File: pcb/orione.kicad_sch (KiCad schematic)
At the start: 187 parts, among them J1 Conn_02x10_Odd_Even, J2 Conn_02x10_Odd_Even

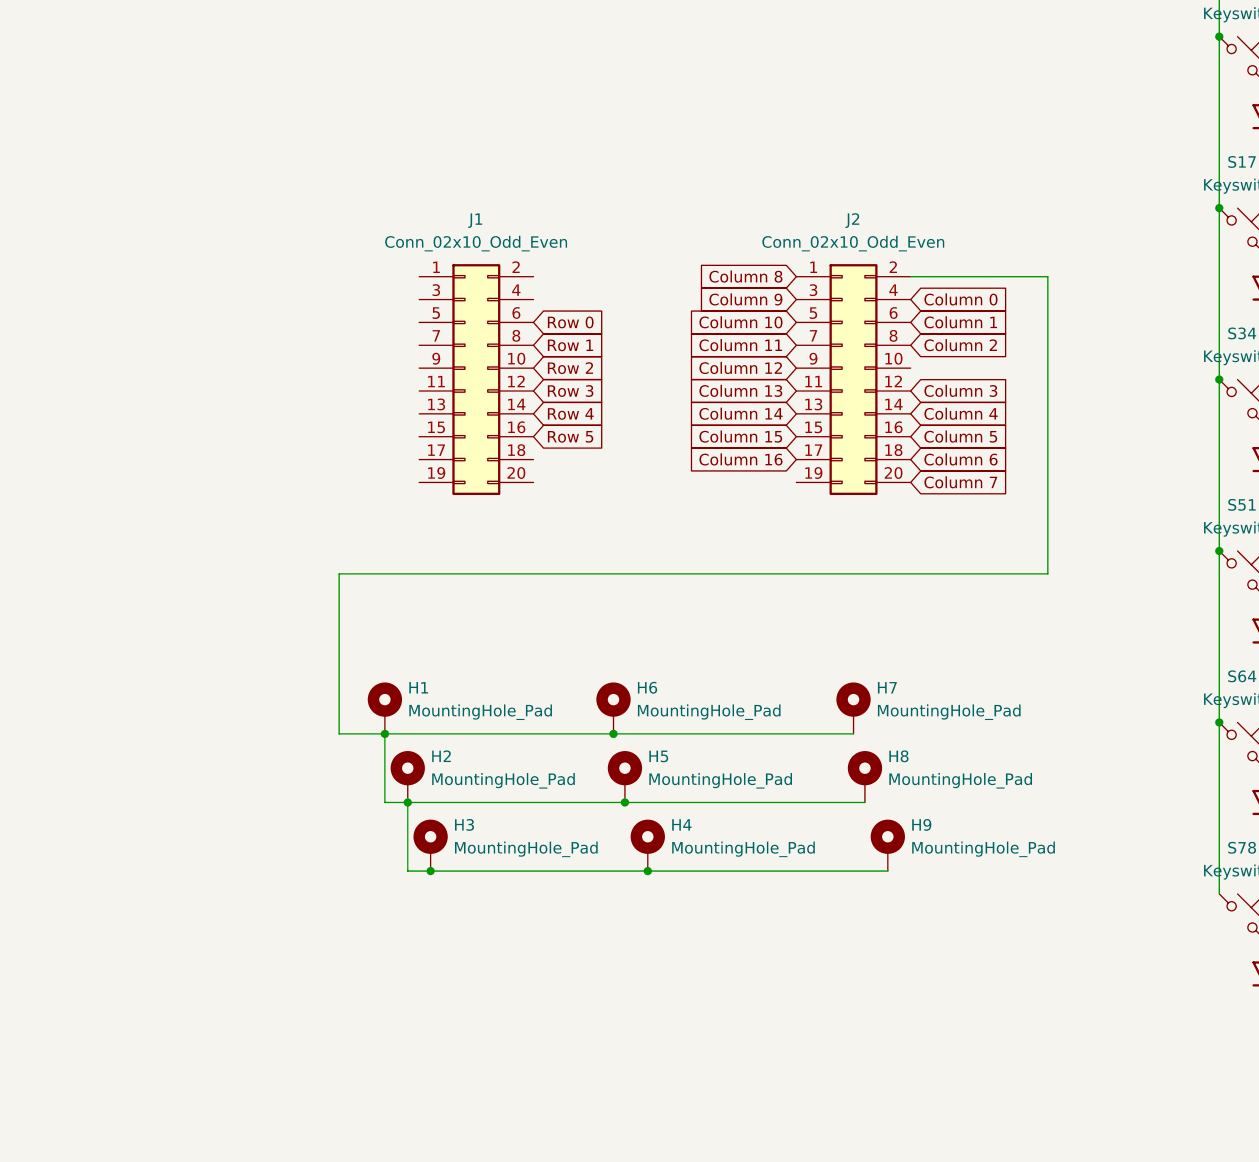
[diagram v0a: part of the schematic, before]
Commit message: minor updtaes to pcb
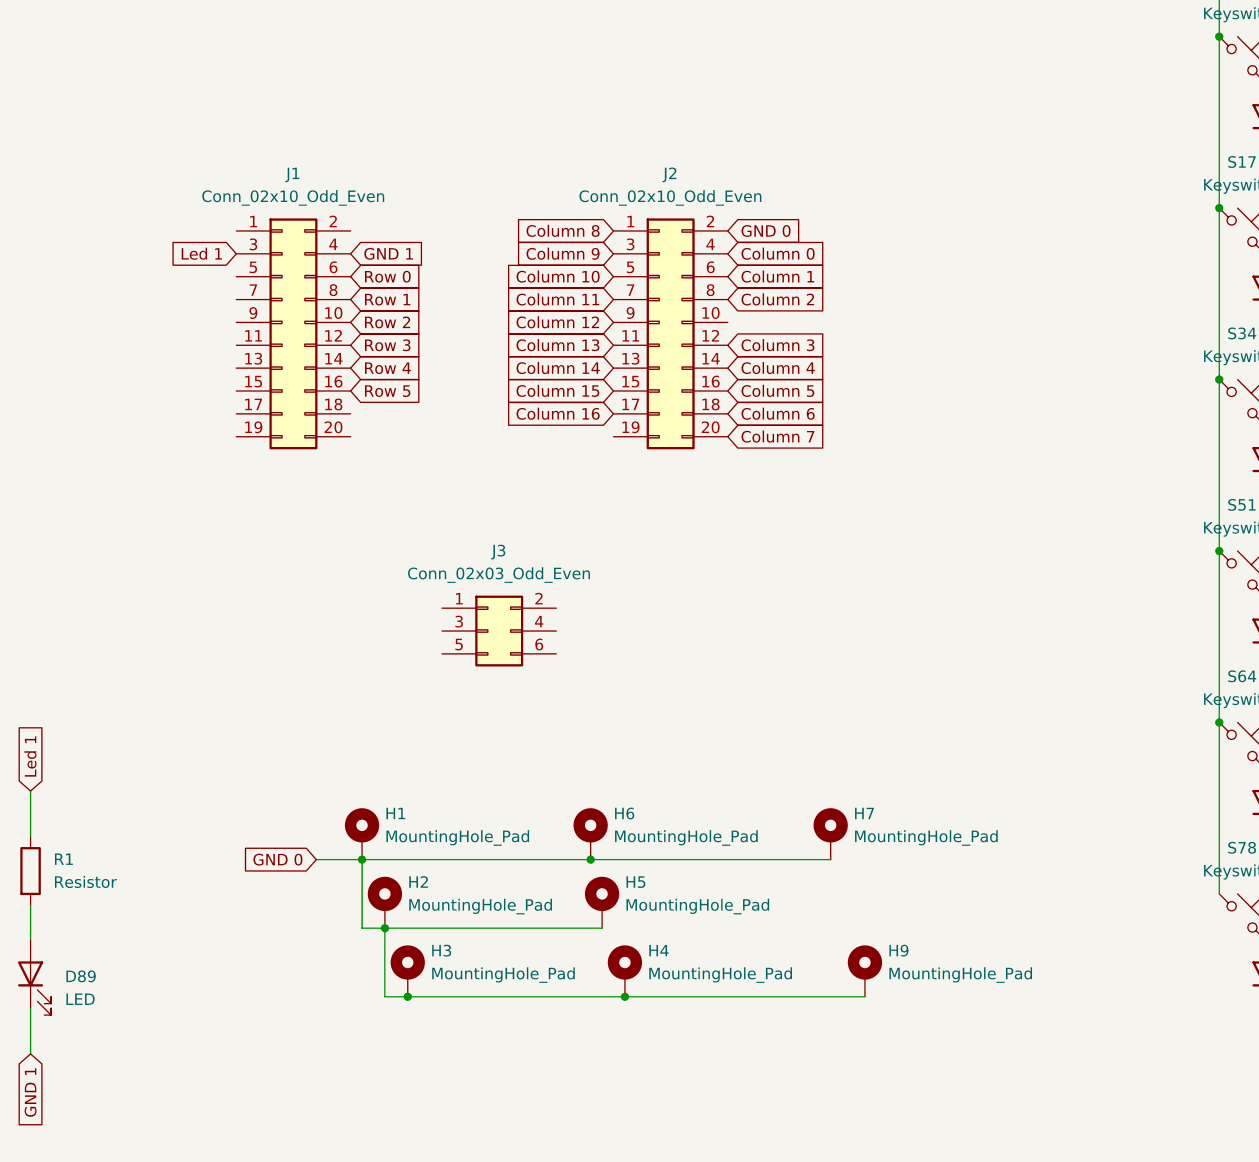
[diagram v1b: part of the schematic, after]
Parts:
- removed H8: MountingHole_Pad, MountingHole:MountingHole_3.2mm_M3_Pad_Via, symbol Mechanical:MountingHole_Pad
- added D89: LED, LED_THT:LED_D5.0mm, symbol Device:LED
- added J3: Conn_02x03_Odd_Even, Connector_PinHeader_2.54mm:PinHeader_2x03_P2.54mm_Horizontal, symbol Connector_Generic:Conn_02x03_Odd_Even
- added R1: Resistor, Resistor_THT:R_Axial_DIN0207_L6.3mm_D2.5mm_P10.16mm_Horizontal, symbol ScottoKeebs:Placeholder_Resistor
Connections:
- net GND 0: now reaches H1.1, H2.1, H3.1, H4.1, H5.1, H6.1, H7.1, H9.1, J2.2 (Pin_2)
- net Led 1: now reaches J1.3 (Pin_3)
- net Led 1: now also R1.1
- net GND 1: now reaches J1.4 (Pin_4)
- net GND 1: now also D89.1 (K)
- new net: D89.2 (A), R1.2
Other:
- moved on the sheet: H1, H2, H3, H4, H5, H6, H7, H9, J1, J2
